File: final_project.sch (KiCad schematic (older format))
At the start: 2 parts, among them J1 Conn_01x02_Female

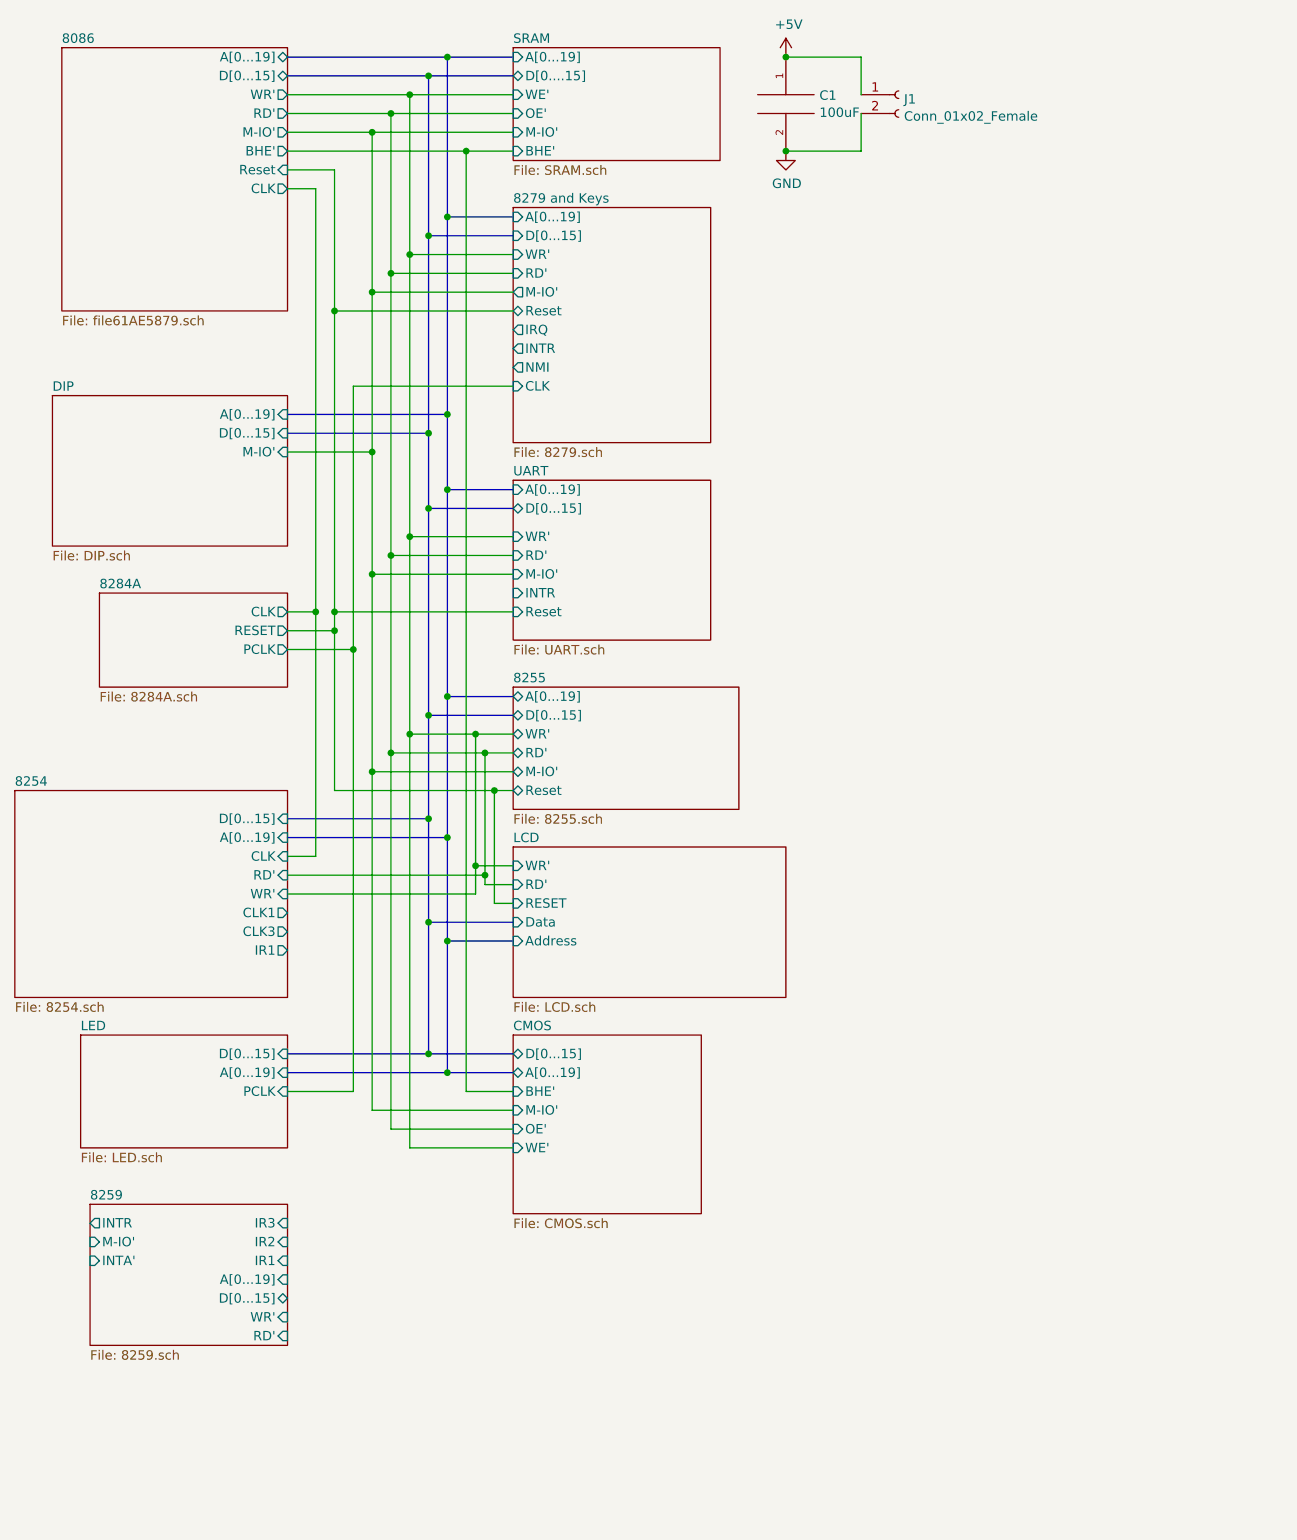
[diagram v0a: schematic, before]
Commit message: Wired Root
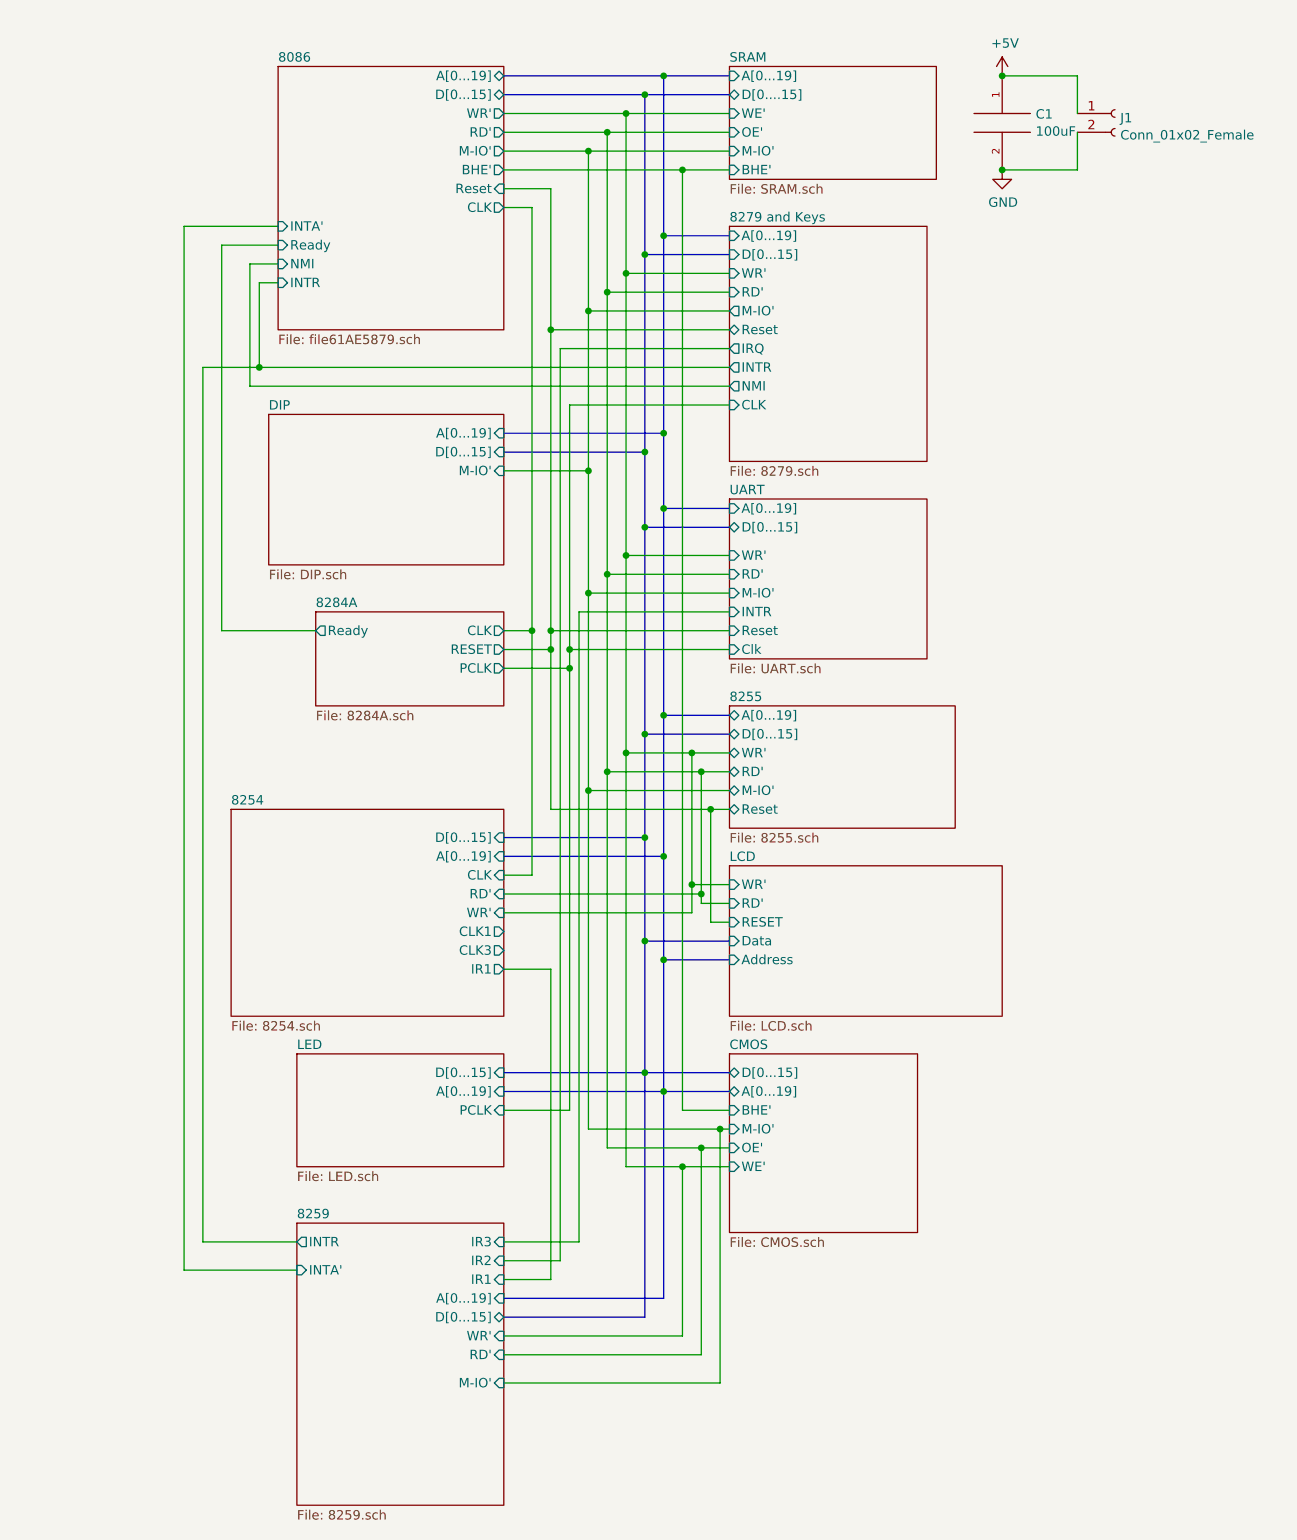
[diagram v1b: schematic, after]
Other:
- moved on the sheet: C1, J1
